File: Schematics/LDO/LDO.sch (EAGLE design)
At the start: 58 parts, among them IC1 LM317MBSTT3, IC2 LM317MBSTT3, Q1 32.768kHz, X1 MINI-USB-SHIELD-UX60-MB-5ST, X2 RJ45

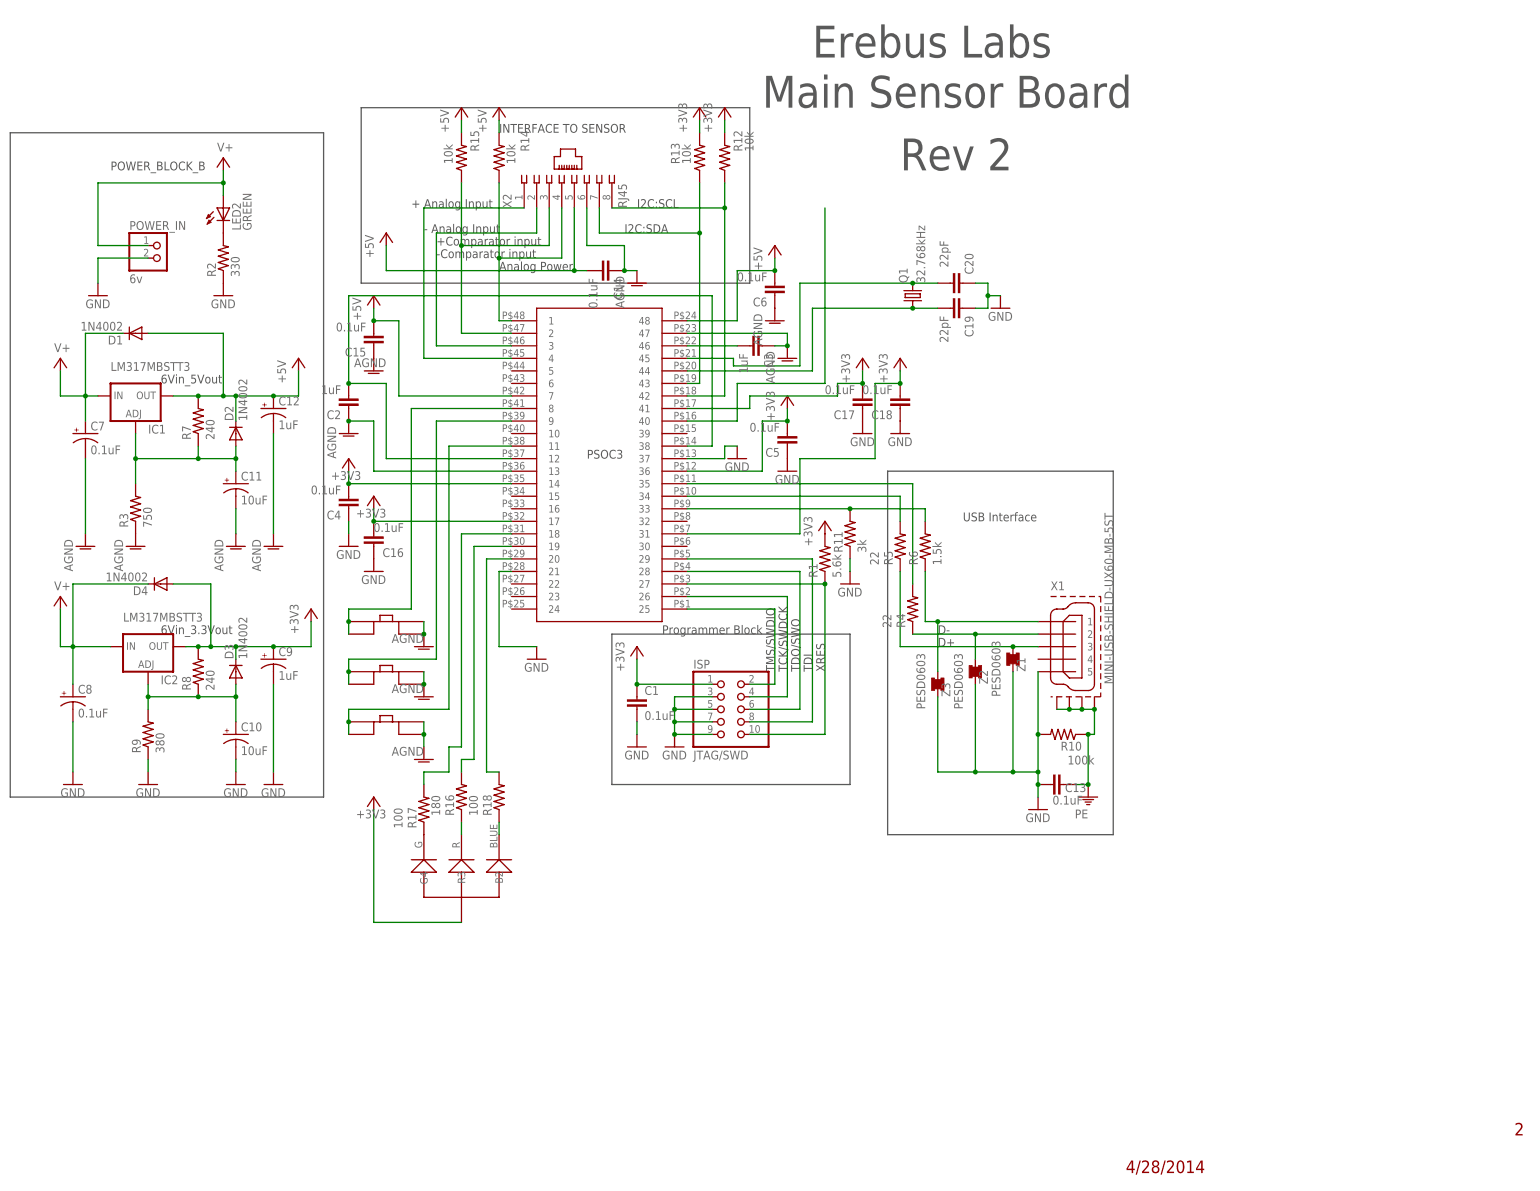
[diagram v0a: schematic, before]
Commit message: Layout Update
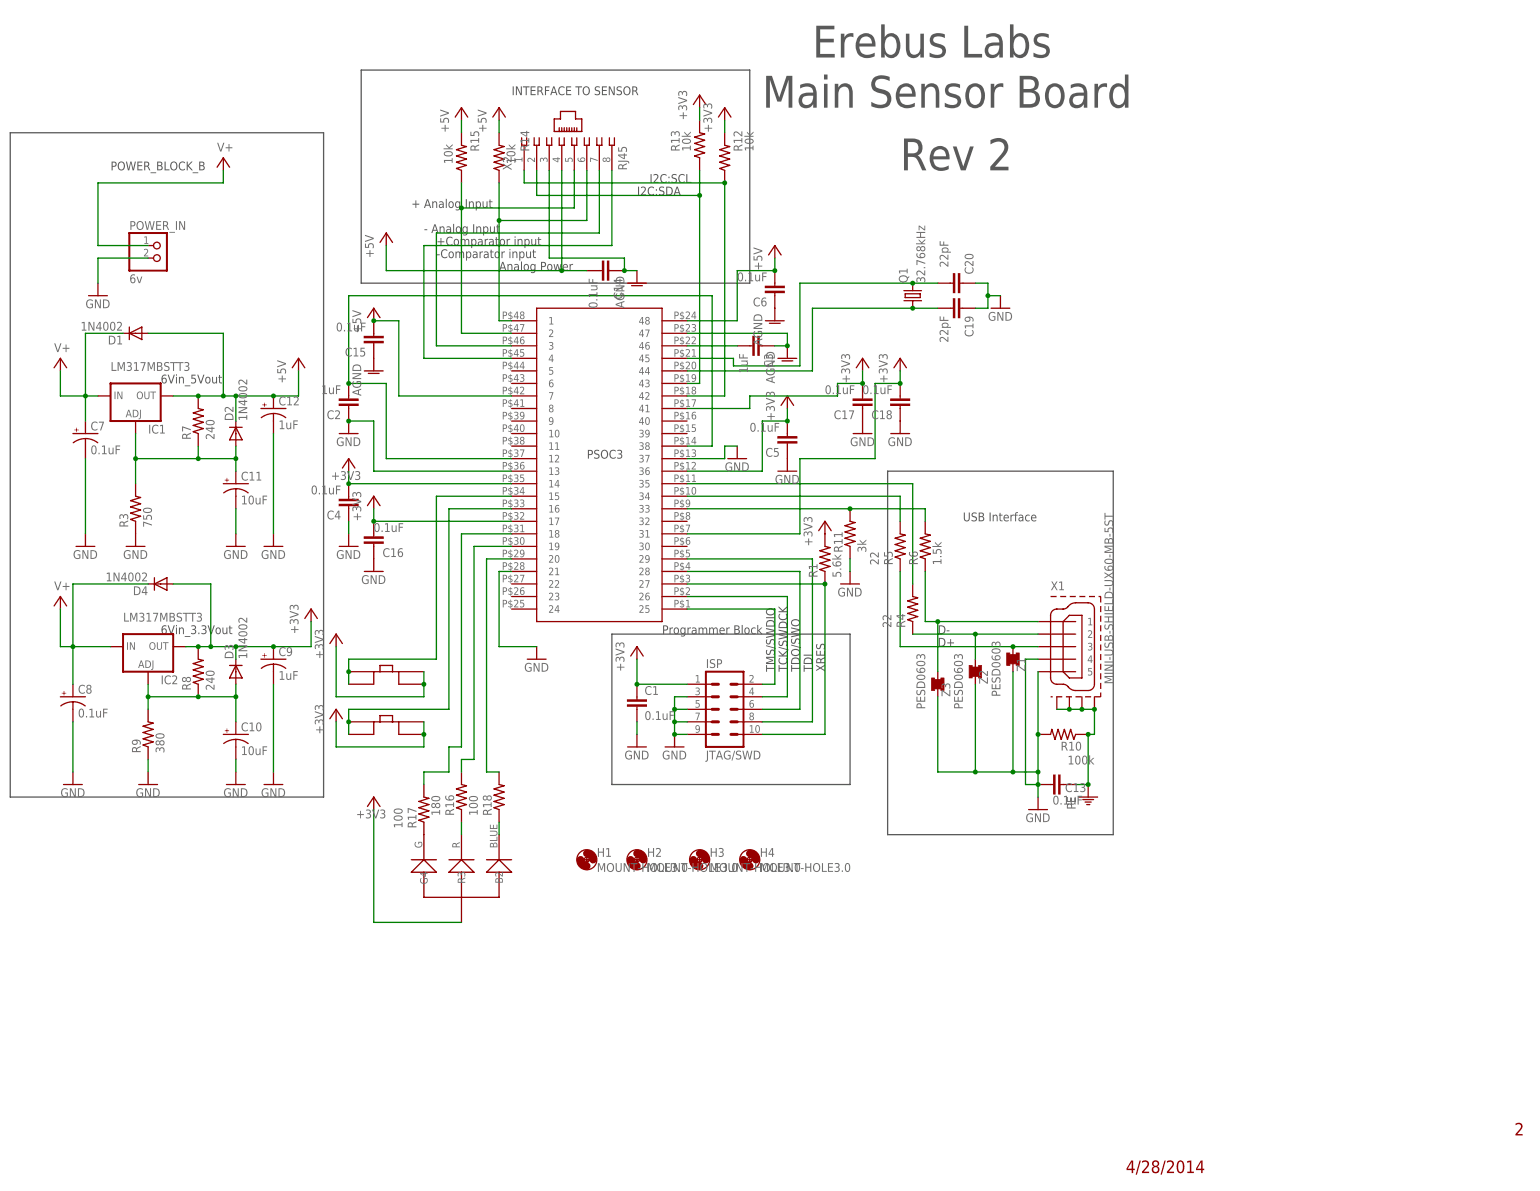
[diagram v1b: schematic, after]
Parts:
- removed LED2: GREEN, led:LED5MM
- removed R2: 330, rcl:R-US_R0603
- removed U$4: SPST, Switches_SPST:SPST
- added H1, H2, H3, H4: MOUNT-HOLE3.0, holes:MOUNT-HOLE3.0
- ISP: device pinhead:PINHD-2X5/90 -> con-samtec:FTSH-105-01-L-DV-K
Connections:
- removed net N$12: LED2.C, R2.2
- removed net N$22: U$1.40
- removed net N$45: U$1.8, U$4.A1, U$4.A2
- new net PE: C13.1, R10.1, X1.GND1, X1.GND2, X1.GND3, X1.GND4
- net +3V3: now also C16.2, U$1.17, U$5.B1, U$5.B2, U$6.B1, U$6.B2
- net +5V: now also X2.4; no longer C16.2, U$1.17, X2.5
- net AGND: now also C14.1, C15.1, C3.1, C6.1, U$1.47, X2.3; no longer C13.1, R10.1, U$4.B1, U$4.B2, U$5.B1, U$5.B2, U$6.B1, U$6.B2, X1.GND1, X1.GND2, X1.GND3, X1.GND4
- net ANALOGINPUT: now also X2.7; no longer X2.2
- net GND: now also X1.4; no longer C14.1, C15.1, C3.1, C6.1, R2.1, U$1.47, X2.6
- net N$18: now also X2.5; no longer X2.3
- net N$19: now also X2.6; no longer X2.4
- net N$20: now also X2.2; no longer X2.7
- net N$21: now also X2.1; no longer X2.8
- net N$41: now also U$1.15; no longer U$1.9
- net N$42: now also X2.8; no longer X2.1
- net N$44: now also U$1.16; no longer U$1.11
- net V+: no longer LED2.A
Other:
- moved on the sheet: R13, X2

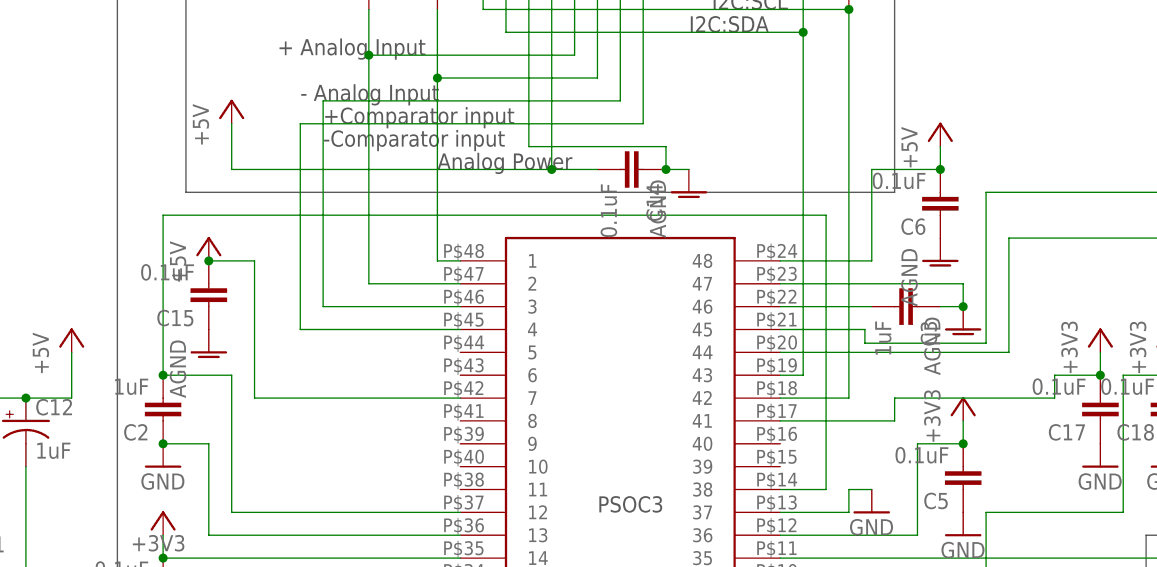
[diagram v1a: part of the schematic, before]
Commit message: LDO Layout
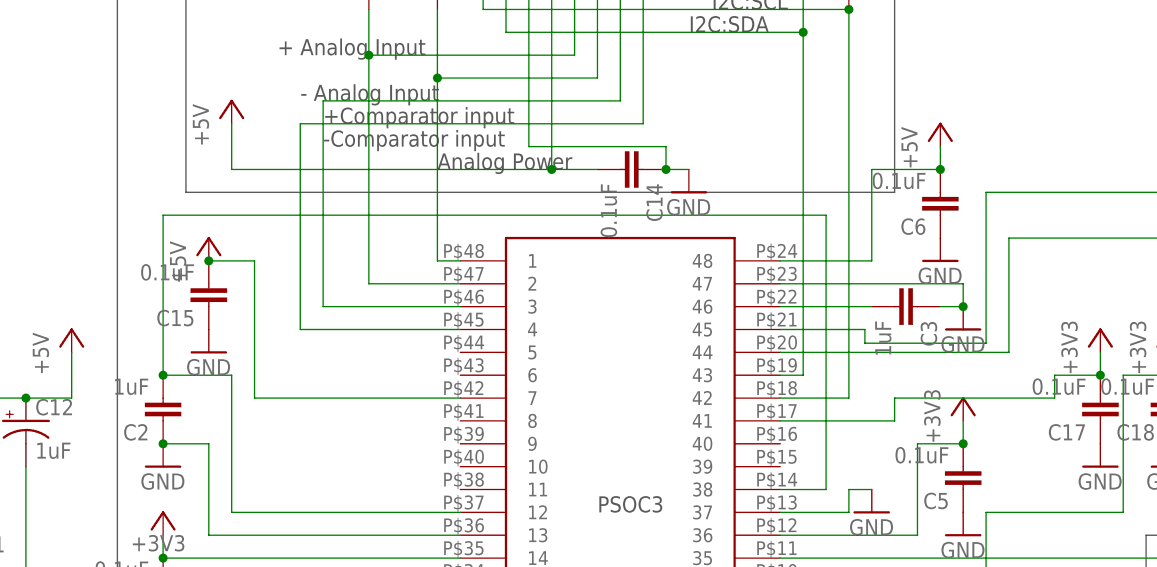
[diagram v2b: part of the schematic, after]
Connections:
- removed net AGND: C14.1, C15.1, C3.1, C6.1, U$1.47, X2.3
- net GND: now also C14.1, C15.1, C3.1, C6.1, U$1.47, X2.3
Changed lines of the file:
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@@
 <part name="+3V12" library="supply1" deviceset="+3V3" device=""/>
 <part name="GND4" library="supply1" deviceset="GND" device=""/>
-<part name="AGND6" library="supply1" deviceset="AGND" device=""/>
-<part name="AGND7" library="supply1" deviceset="AGND" device=""/>
-<part name="AGND8" library="supply1" deviceset="AGND" device=""/>
 <part name="PE1" library="supply1" deviceset="PE" device=""/>
-<part name="AGND1" library="supply1" deviceset="AGND" device=""/>
 <part name="GND6" library="supply1" deviceset="GND" device=""/>
 <part name="GND10" library="supply1" deviceset="GND" device=""/>
@@
 <part name="H3" library="holes" deviceset="MOUNT-HOLE" device="3.0"/>
 <part name="H4" library="holes" deviceset="MOUNT-HOLE" device="3.0"/>
+<part name="GND14" library="supply1" deviceset="GND" device=""/>
+<part name="GND15" library="supply1" deviceset="GND" device=""/>
+<part name="GND16" library="supply1" deviceset="GND" device=""/>
+<part name="GND21" library="supply1" deviceset="GND" device=""/>
 </parts>
 <sheets>
@@
 <instance part="+3V12" gate="G$1" x="-17.78" y="45.72"/>
 <instance part="GND4" gate="1" x="-22.86" y="58.42"/>
-<instance part="AGND6" gate="VR1" x="35.56" y="88.9"/>
-<instance part="AGND7" gate="VR1" x="63.5" y="81.28"/>
-<instance part="AGND8" gate="VR1" x="66.04" y="73.66"/>
 <instance part="PE1" gate="M" x="127" y="-15.24"/>
-<instance part="AGND1" gate="VR1" x="-17.78" y="71.12"/>
 <instance part="GND6" gate="1" x="-38.1" y="35.56"/>
 <instance part="GND10" gate="1" x="-45.72" y="35.56"/>
@@
 <instance part="H3" gate="G$1" x="48.26" y="-27.94"/>
 <instance part="H4" gate="G$1" x="58.42" y="-27.94"/>
+<instance part="GND14" gate="1" x="-17.78" y="71.12"/>
+<instance part="GND15" gate="1" x="35.56" y="88.9"/>
+<instance part="GND16" gate="1" x="66.04" y="73.66"/>
+<instance part="GND21" gate="1" x="63.5" y="81.28"/>
 </instances>
 <busses>
@@
 <pinref part="GND13" gate="1" pin="GND"/>
 </segment>
+<segment>
+<pinref part="C15" gate="G$1" pin="1"/>
+<pinref part="GND14" gate="1" pin="GND"/>
+</segment>
+<segment>
+<pinref part="C14" gate="G$1" pin="1"/>
+<wire x1="35.56" y1="91.44" x2="33.02" y2="91.44" width="0.1524" layer="91"/>
+<pinref part="X2" gate="G$1" pin="3"/>
+<wire x1="17.78" y1="111.76" x2="17.78" y2="93.98" width="0.1524" layer="91"/>
+<wire x1="17.78" y1="93.98" x2="33.02" y2="93.98" width="0.1524" layer="91"/>
+<wire x1="33.02" y1="93.98" x2="33.02" y2="91.44" width="0.1524" layer="91"/>
+<junction x="33.02" y="91.44"/>
+<pinref part="GND15" gate="1" pin="GND"/>
+</segment>
+<segment>
+<pinref part="U$1" gate="G$1" pin="47"/>
+<wire x1="45.72" y1="78.74" x2="66.04" y2="78.74" width="0.1524" layer="91"/>
+<wire x1="66.04" y1="78.74" x2="66.04" y2="76.2" width="0.1524" layer="91"/>
+<pinref part="C3" gate="G$1" pin="1"/>
+<wire x1="66.04" y1="76.2" x2="63.5" y2="76.2" width="0.1524" layer="91"/>
+<pinref part="GND16" gate="1" pin="GND"/>
+<junction x="66.04" y="76.2"/>
+</segment>
+<segment>
+<pinref part="C6" gate="G$1" pin="1"/>
+<pinref part="GND21" gate="1" pin="GND"/>
+</segment>
 </net>
 <net name="N$11" class="0">
@@
 </segment>
 </net>
-<net name="AGND" class="0">
-<segment>
-<pinref part="C14" gate="G$1" pin="1"/>
-<wire x1="35.56" y1="91.44" x2="33.02" y2="91.44" width="0.1524" layer="91"/>
-<pinref part="AGND6" gate="VR1" pin="AGND"/>
-<pinref part="X2" gate="G$1" pin="3"/>
-<wire x1="17.78" y1="111.76" x2="17.78" y2="93.98" width="0.1524" layer="91"/>
-<wire x1="17.78" y1="93.98" x2="33.02" y2="93.98" width="0.1524" layer="91"/>
-<wire x1="33.02" y1="93.98" x2="33.02" y2="91.44" width="0.1524" layer="91"/>
-<junction x="33.02" y="91.44"/>
-</segment>
-<segment>
-<pinref part="C6" gate="G$1" pin="1"/>
-<pinref part="AGND7" gate="VR1" pin="AGND"/>
-</segment>
-<segment>
-<pinref part="U$1" gate="G$1" pin="47"/>
-<wire x1="45.72" y1="78.74" x2="66.04" y2="78.74" width="0.1524" layer="91"/>
-<wire x1="66.04" y1="78.74" x2="66.04" y2="76.2" width="0.1524" layer="91"/>
-<pinref part="C3" gate="G$1" pin="1"/>
-<wire x1="66.04" y1="76.2" x2="63.5" y2="76.2" width="0.1524" layer="91"/>
-<pinref part="AGND8" gate="VR1" pin="AGND"/>
-<junction x="66.04" y="76.2"/>
-</segment>
-<segment>
-<pinref part="C15" gate="G$1" pin="1"/>
-<pinref part="AGND1" gate="VR1" pin="AGND"/>
-</segment>
-</net>
